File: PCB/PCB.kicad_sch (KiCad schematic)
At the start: 41 parts, among them J1 USB_C_Receptacle_USB2.0_14P, J2 OLED_128x64, SW1 SW_Push, SW2 RotaryEncoder, SW3 RotaryEncoder, U1 STM32F072CBTx, U2 USBLC6-2SC6, U3 XC6206, U5 TRRS

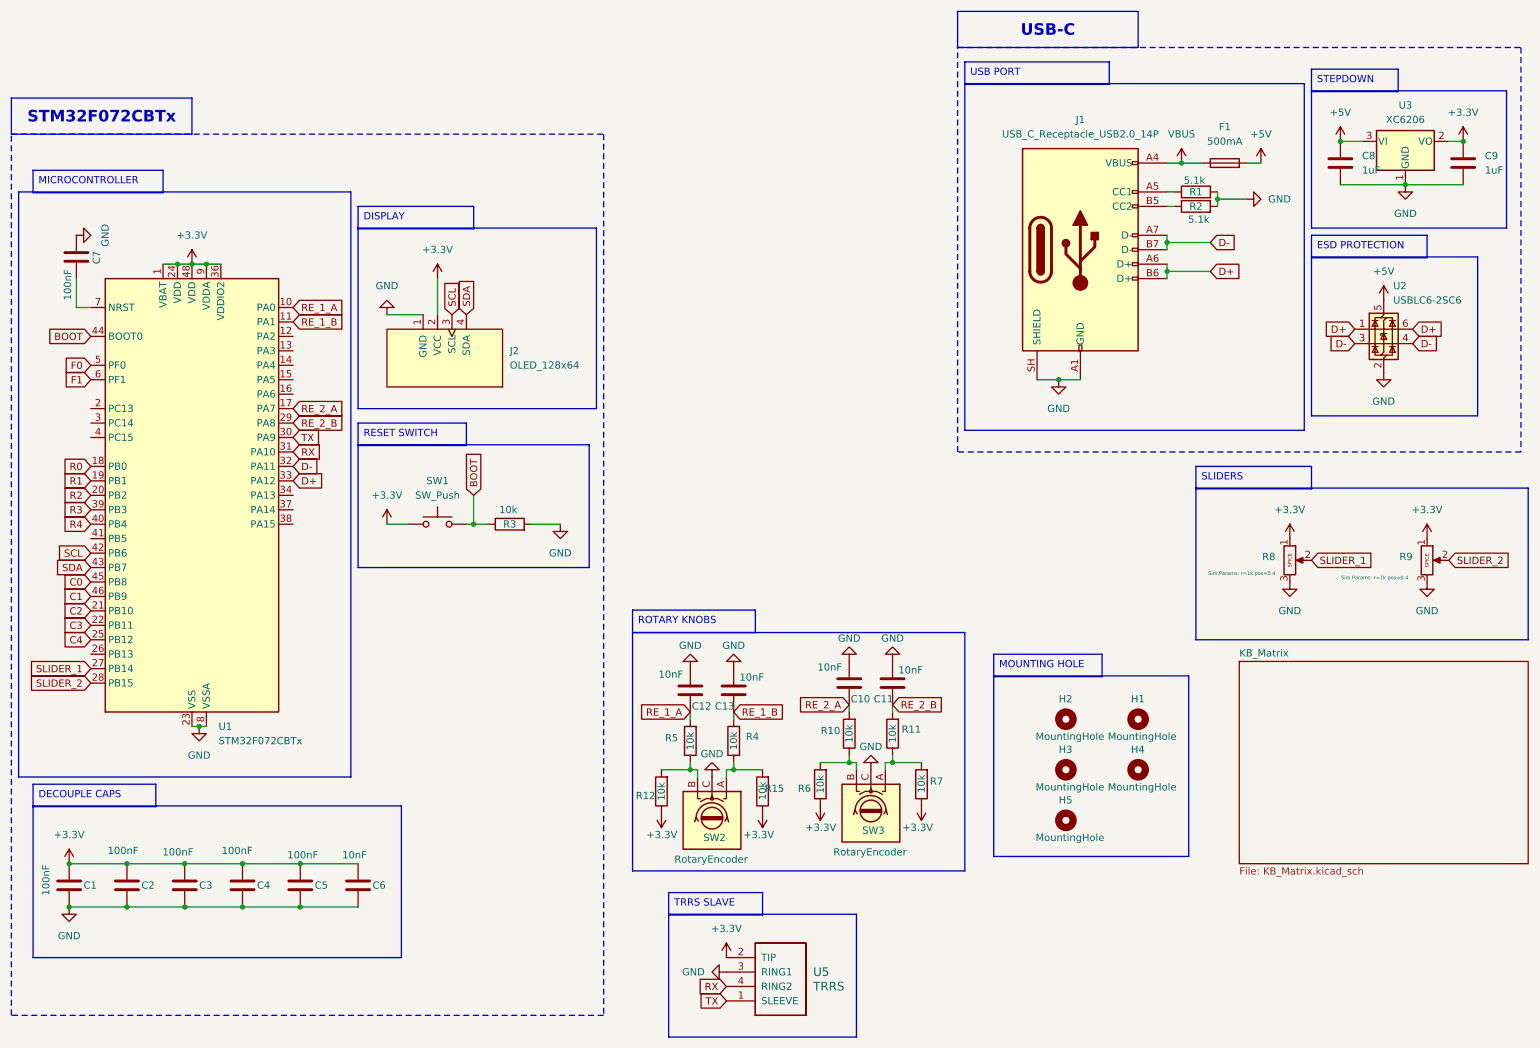
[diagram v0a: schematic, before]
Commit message: Updated
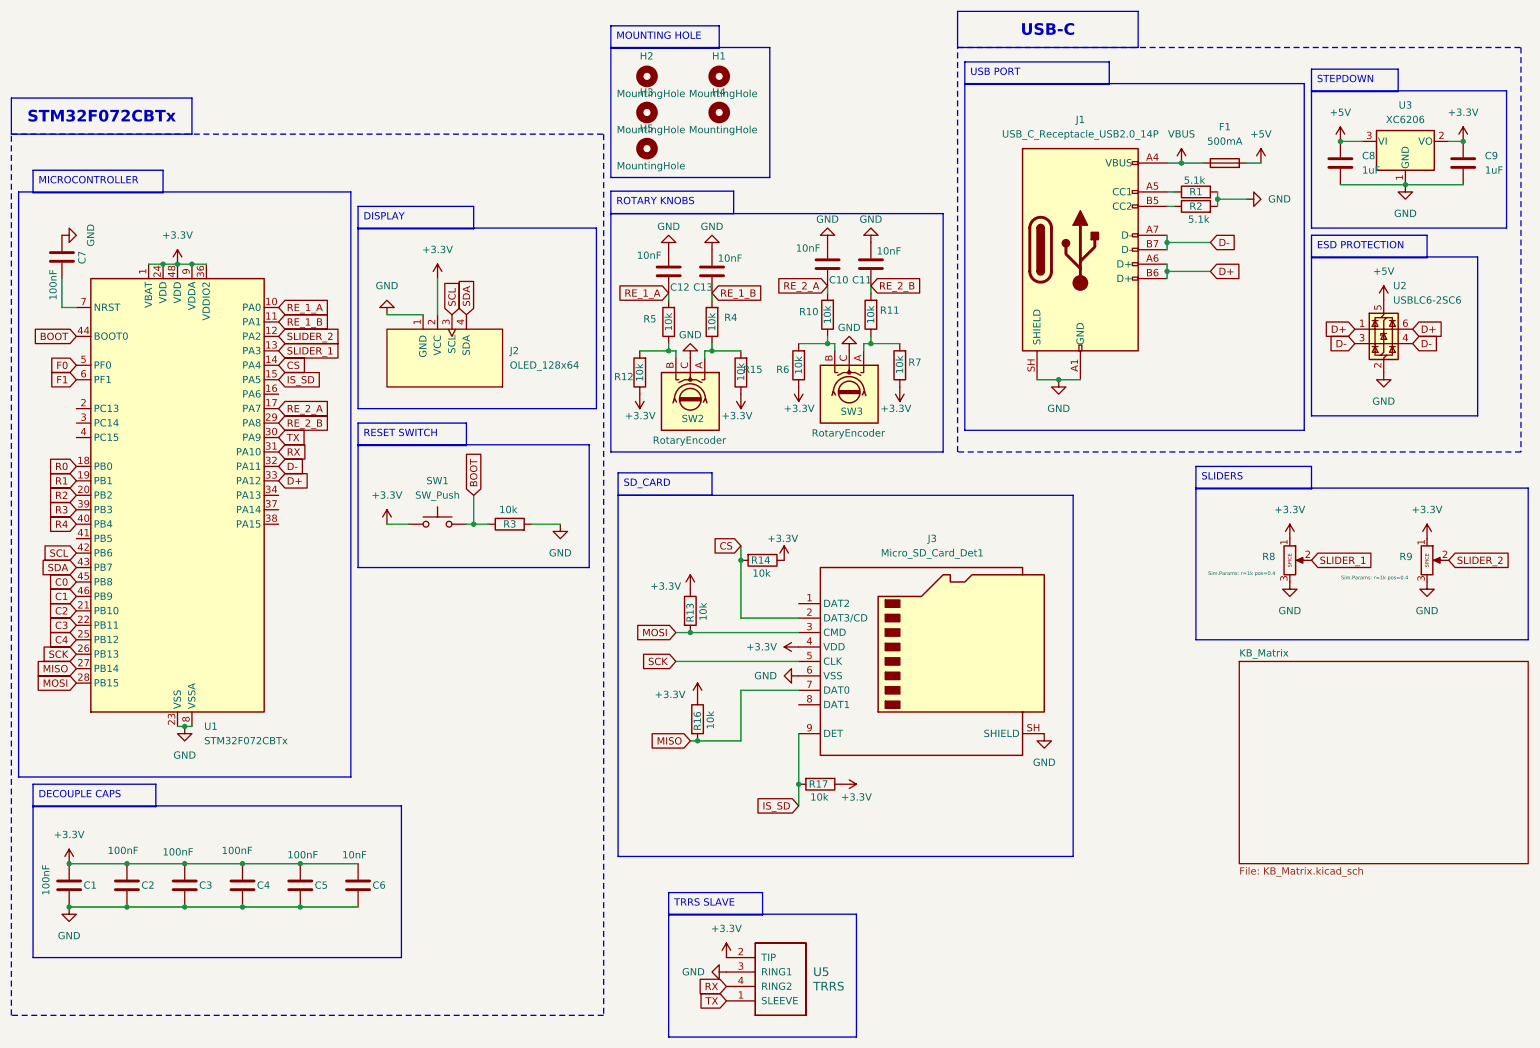
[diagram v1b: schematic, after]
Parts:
- added J3: Micro_SD_Card_Det1, symbol Connector:Micro_SD_Card_Det1
- added R13, R14, R16, R17: 10k, symbol Device:R
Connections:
- net +3.3V: now also J3.4 (VDD), R13.1, R14.1, R16.1, R17.1
- net GND: now also J3.6 (VSS), J3.SH (SHIELD)
- net SLIDER_1: now also U1.13 (PA3); no longer U1.27 (PB14)
- net SLIDER_2: now also U1.12 (PA2); no longer U1.28 (PB15)
- net CS: now reaches U1.14 (PA4)
- net CS: now also J3.2 (DAT3/CD), R14.2
- net IS_SD: now reaches U1.15 (PA5)
- net IS_SD: now also J3.9 (DET), R17.2
- net SCK: now reaches U1.26 (PB13)
- net SCK: now also J3.5 (CLK)
- new net MISO: J3.7 (DAT0), R16.2, U1.27 (PB14)
- new net MOSI: J3.3 (CMD), R13.2, U1.28 (PB15)
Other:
- moved on the sheet: C7, H1, H2, H3, H4, H5, U1
